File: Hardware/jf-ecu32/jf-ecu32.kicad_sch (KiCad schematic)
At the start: 31 parts, among them J1 GAZ, J10 k, J11 RPM, J12 S.PORT, J2 AUX, J3 PPM/PWM, J4 STARTER, J5 GLOW, J6 VANNE KEROSTART, J7 VANNE KERO, J8 BATTERY 2S/3S, J9 STARTER, Q1 QM6006D, Q2 QM6006D, Q3 QM6006D, Q4 QM6006D, U1 ESP32-DevKitC, U2 4050, U3 MAX31855KASA, U4 AMS1117-3.3, U5 4050

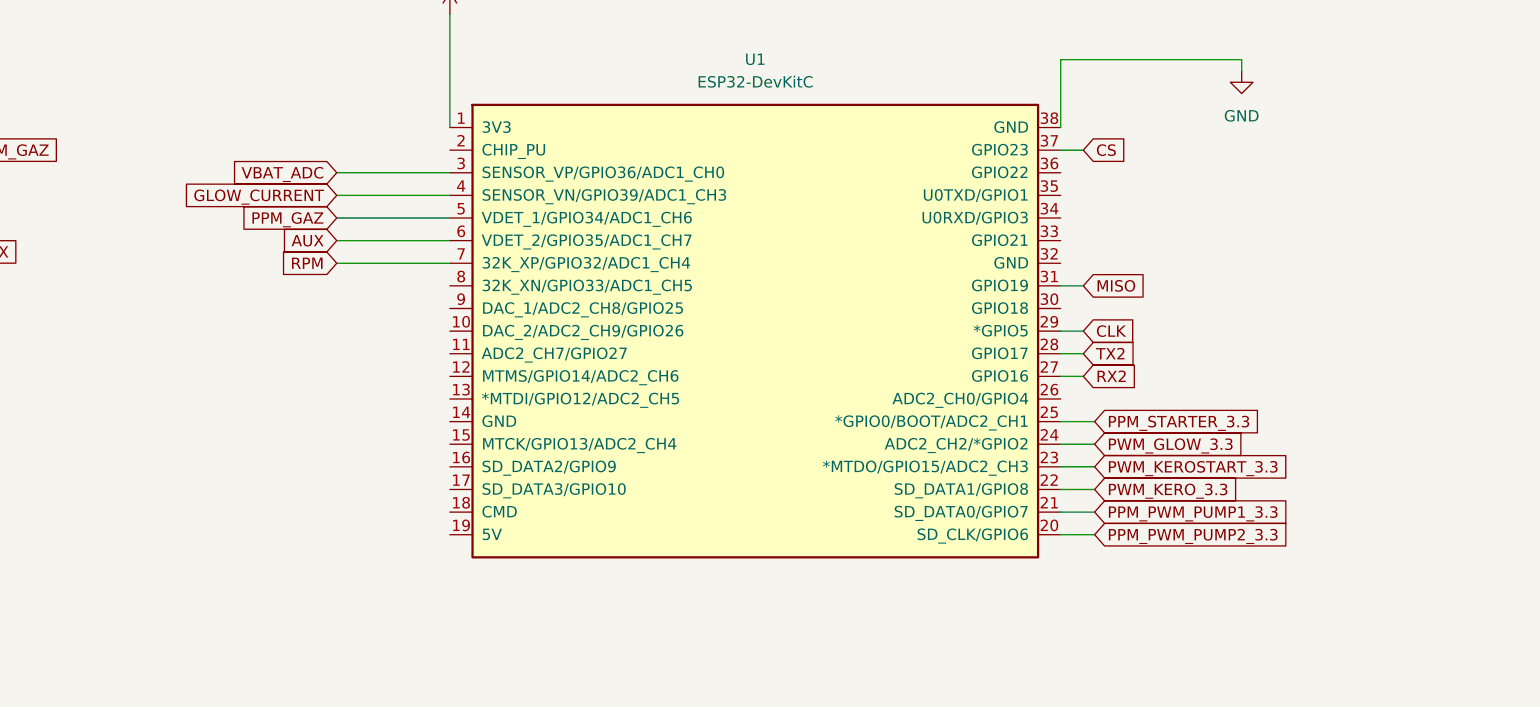
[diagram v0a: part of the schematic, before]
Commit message: update
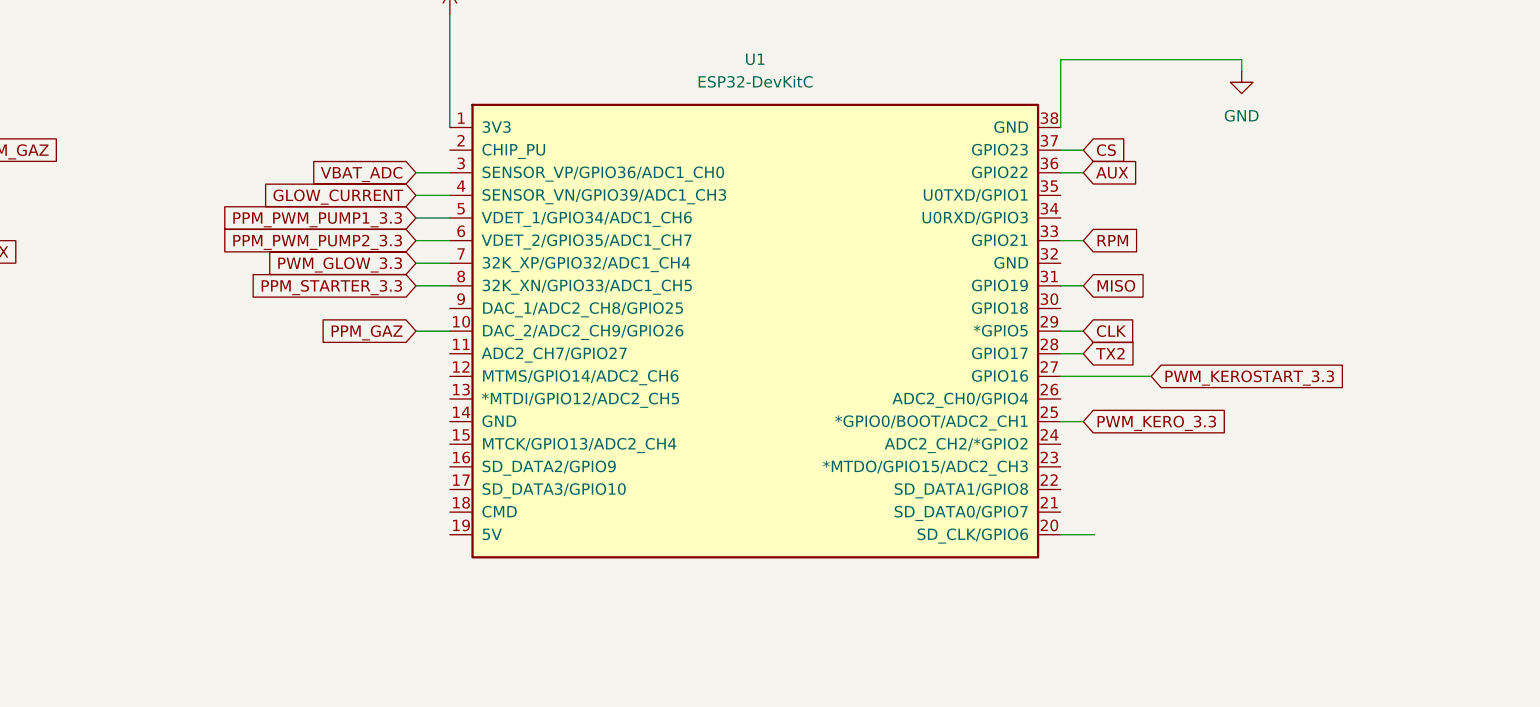
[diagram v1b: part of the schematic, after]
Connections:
- net RX2 is gone; now on net PWM_KEROSTART_3.3: U1.27 (GPIO16)
- net AUX: now also U1.36 (GPIO22); no longer U1.6 (VDET_2/GPIO35/ADC1_CH7)
- net PPM_GAZ: now also U1.10 (DAC_2/ADC2_CH9/GPIO26); no longer U1.5 (VDET_1/GPIO34/ADC1_CH6)
- net PPM_PWM_PUMP1_3.3: now also U1.5 (VDET_1/GPIO34/ADC1_CH6); no longer U1.21 (SD_DATA0/GPIO7)
- net PPM_PWM_PUMP2_3.3: now also U1.6 (VDET_2/GPIO35/ADC1_CH7); no longer U1.20 (SD_CLK/GPIO6)
- net PPM_STARTER_3.3: now also U1.8 (32K_XN/GPIO33/ADC1_CH5); no longer U1.25 (*GPIO0/BOOT/ADC2_CH1)
- net PWM_GLOW_3.3: now also U1.7 (32K_XP/GPIO32/ADC1_CH4); no longer U1.24 (ADC2_CH2/*GPIO2)
- net PWM_KEROSTART_3.3: no longer U1.23 (*MTDO/GPIO15/ADC2_CH3)
- net PWM_KERO_3.3: now also U1.25 (*GPIO0/BOOT/ADC2_CH1); no longer U1.22 (SD_DATA1/GPIO8)
- net RPM: now also U1.33 (GPIO21); no longer U1.7 (32K_XP/GPIO32/ADC1_CH4)
